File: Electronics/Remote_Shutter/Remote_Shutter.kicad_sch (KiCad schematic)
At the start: 8 parts

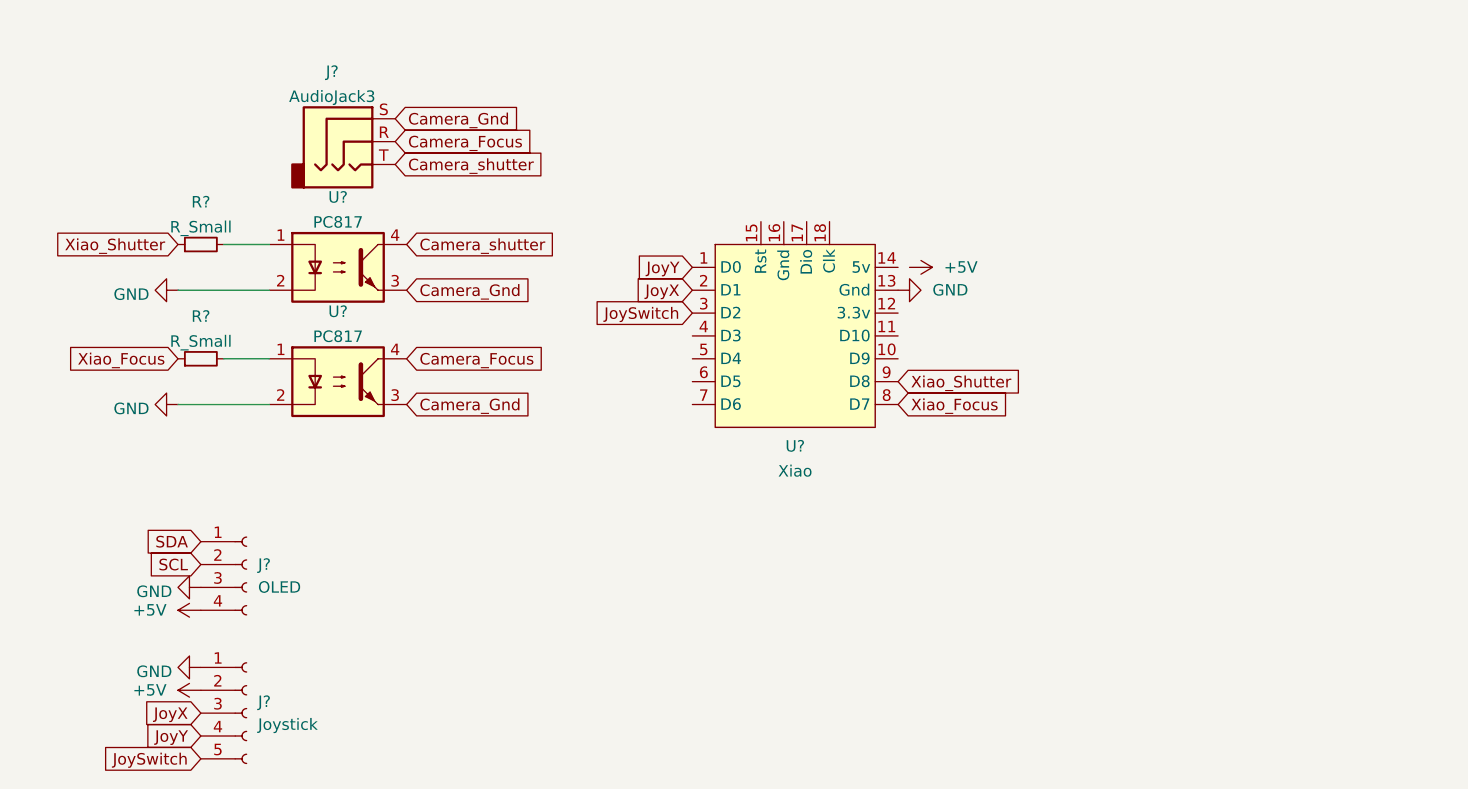
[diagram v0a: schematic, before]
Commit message: Mostly finished the circuit diagram
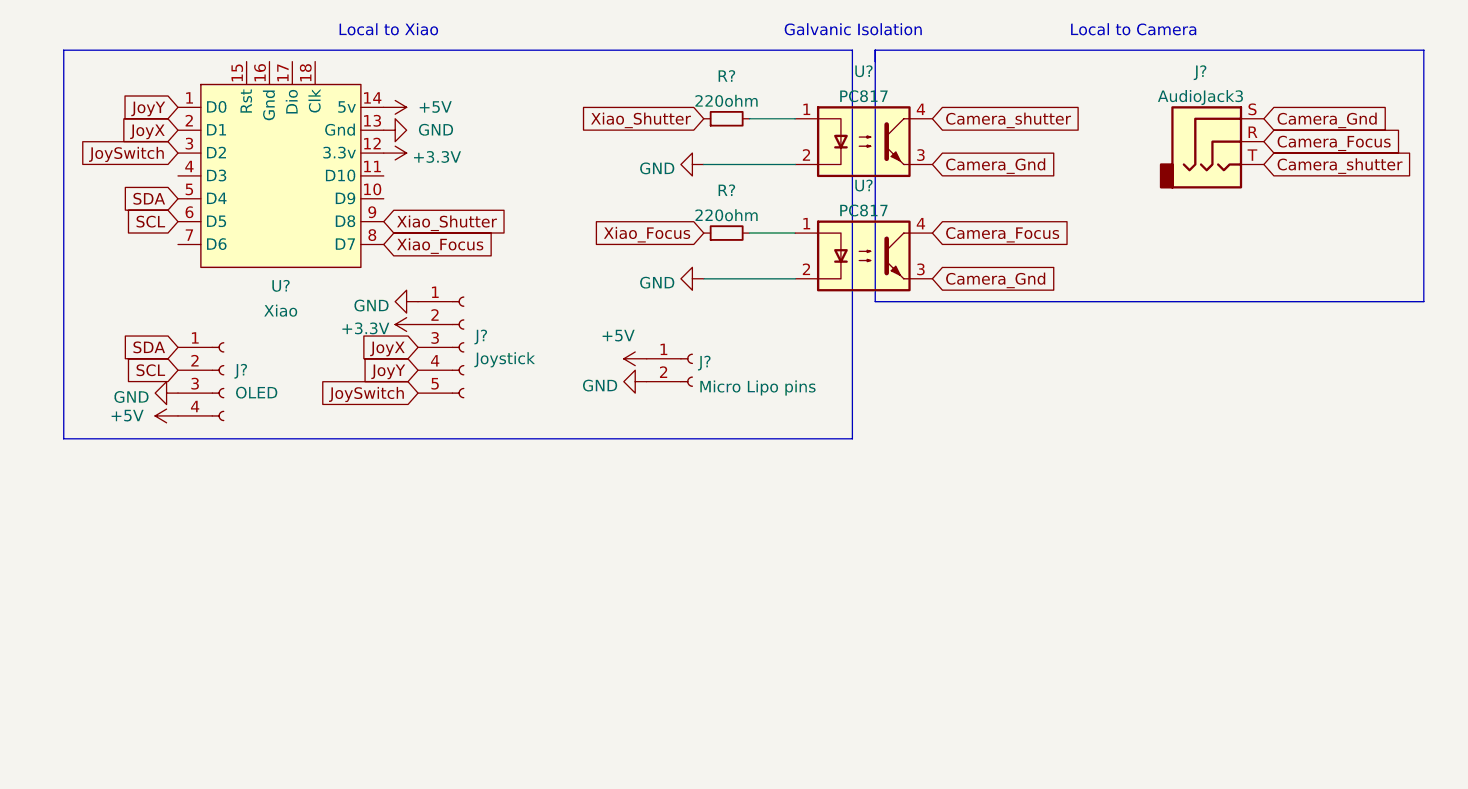
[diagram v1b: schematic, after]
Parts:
- added J?: Micro Lipo pins, symbol Connector:Conn_01x02_Female
- R? (x2): value R_Small -> 220ohm
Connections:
- net +5V: now also U?.14 (5v), J?.1 (Pin_1); no longer J?.2 (Pin_2)
- net GND: now also J?.2 (Pin_2)
- net SCL: now also U?.6 (D5)
- net SDA: now also U?.5 (D4)
- net +3V3: now reaches U?.12 (3.3v)
- net +3V3: now also J?.2 (Pin_2)
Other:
- note added: "Galvanic Isolation"
- note added: "Local to Camera"
- note added: "Local to Xiao"
- moved on the sheet: J?, R?, U?
